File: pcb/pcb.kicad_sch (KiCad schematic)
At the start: 7 parts

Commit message: Start schematic
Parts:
- removed C? (x2): 100n, Capacitor_SMD:C_0603_1608Metric, symbol Device:C
- removed C? (x2): 22u, Capacitor_SMD:CP_Elec_4x3.9, symbol Device:C_Polarized_Small
- removed J?: EURO_PWR_2x5, Connector_IDC:IDC-Header_2x05_P2.54mm_Vertical, symbol eurocad:EURO_PWR_2x5
- removed R? (x2): 22R, Resistor_SMD:R_0603_1608Metric, symbol Device:R
- added C10, C12, C4, C5, C9: 100n, Capacitor_SMD:C_0603_1608Metric, symbol Device:C
- added C11, C13, C2, C3, C6: 10u, Capacitor_SMD:C_0805_2012Metric, symbol Device:C
- added C14, C16: 1n, Capacitor_SMD:C_0603_1608Metric, symbol Device:C
- added C15, C17: 100p, Capacitor_SMD:C_0603_1608Metric, symbol Device:C
- added C7, C8: 2.2u, Capacitor_SMD:C_0805_2012Metric, symbol Device:C
- added D1, D2: 1N5819, Diode_SMD:D_SOD-123, symbol Diode:1N5819
- added D10, D11, D12, D13, D14, D15, D16, D17, D18, D3, D4, D5, D6, D7, D8, D9: BAT54J, Diode_SMD:D_SOD-323F, symbol Diode:BAT54J
- added FB1: BLM21PG600SN1D, Inductor_SMD:L_0805_2012Metric, symbol Device:FerriteBead
- added J1, J10, J11, J2, J3, J5, J6, J7, J8, J9: PJ301M-12, Eurocad:PJ301M-12, symbol eurocad:PJ301M-12
- added J4: EURO_PWR_2x5, Eurocad:Eurorack_Power_Header, symbol eurocad:EURO_PWR_2x5
- added R10, R12, R14, R16, R18, R20, R6, R8: 100K, Resistor_SMD:R_0603_1608Metric, symbol Device:R
- added R11, R13, R15, R17, R19, R21, R25, R29, R7, R9: 1K, Resistor_SMD:R_0603_1608Metric, symbol Device:R
- added R22, R26: 2K2, Resistor_SMD:R_0603_1608Metric, symbol Device:R
- added R23, R27: 10K, Resistor_SMD:R_0603_1608Metric, symbol Device:R
- added R24, R28: 33K, Resistor_SMD:R_0603_1608Metric, symbol Device:R
- added SW1: RotaryEncoder_Switch, Rotary_Encoder:RotaryEncoder_Bourns_Horizontal_PEC09-2xxxF-Nxxxx, symbol Device:RotaryEncoder_Switch
- added U1: PCM5102, Package_SO:TSSOP-20_4.4x6.5mm_P0.65mm, symbol Audio:PCM5102
- added U2: TL072, Package_SO:SOIC-8_3.9x4.9mm_P1.27mm, symbol Amplifier_Operational:TL072
- added U6: Pico, MCU_RaspberryPi_and_Boards:RPi_Pico_SMD_TH, symbol MCU_RaspberryPi_and_Boards:Pico
- added U7: AZ1117-5.0, Package_TO_SOT_SMD:SOT-223-3_TabPin2, symbol Regulator_Linear:AZ1117-5.0
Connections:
- net +12V: now also C2.1, C4.1, D1.1 (K), U2.8 (V+), U7.3 (VI)
- net -12V: now also C3.2, C5.2, D2.2 (A), U2.4 (V-)
- net GND: now also C10.2, C11.2, C12.2, C13.2, C14.2, C16.2, C2.2, C3.1, C4.2, C5.1, C6.2, C8.2, C9.2, D10.2 (A), D12.2 (A), D14.2 (A), D16.2 (A), D18.2 (A), D3.2 (A), D6.2 (A), D8.2 (A), J1.1, J10.1, J11.1, J2.1, J3.1, J4.3 (GND), J4.4 (GND), J4.5 (GND), J4.6 (GND), J4.7 (GND), J4.8 (GND), J5.1, J6.1, J7.1, J8.1, J9.1, R10.1, R12.1, R14.1, R16.1, R18.1, R20.1, R6.1, R8.1, U1.10 (DEMP), U1.11 (FLT), U1.12 (SCK), U1.16 (FMT), U1.19 (DGND), U1.3 (CPGND), U1.9 (AGND), U2.3 (+), U2.5 (+), U6.13 (GND), U6.18 (GND), U6.23 (GND), U6.28 (GND), U6.3 (GND), U6.33 (AGND), U6.38 (GND), U6.42 (GND), U6.8 (GND), U7.1 (GND)
- new net: J2.3, R8.2, R9.2
- new net: C7.1, U1.2 (CAPP)
- new net: C7.2, U1.4 (CAPM)
- new net: C10.1, C11.1, FB1.2, U1.1 (CPVDD), U1.8 (AVDD)
- new net: J8.3, R18.2, R19.2
- new net: J7.3, R16.2, R17.2
- new net: C17.1, R27.1, R28.2, U2.6 (-)
- new net: C17.2, R28.1, R29.2, U2.7
- new net: C9.1, U1.18 (LDOO)
- new net: C8.1, U1.5 (VNEG)
- new net: J6.3, R14.2, R15.2
- new net: J3.3, R10.2, R11.2
- new net: J9.3, R20.2, R21.2
- new net: D1.2 (A), J4.1 (+12V), J4.2 (+12V)
- new net: D2.1 (K), J4.10 (-12V), J4.9 (-12V)
- new net: J5.3, R12.2, R13.2
- new net: C15.2, R24.1, R25.2, U2.1
- new net: C15.1, R23.1, R24.2, U2.2 (-)
- new net: C14.1, R22.1, R23.2
- new net: J11.3, R29.1
- new net: J10.3, R25.1
- new net: C16.1, R26.1, R27.2
- new net: J1.3, R6.2, R7.2
- new net +3V3: C12.1, C13.1, D11.1 (K), D13.1 (K), D15.1 (K), D17.1 (K), D4.1 (K), D5.1 (K), D7.1 (K), D9.1 (K), FB1.1, U1.20 (DVDD), U6.36 (3V3)
- new net +5V: C6.1, U6.39 (VSYS), U7.2 (VO)
- new net GPIO26: U1.14 (DIN), U6.31 (GPIO26_ADC0)
- new net GPIO27: U1.13 (BCK), U6.32 (GPIO27_ADC1)
- new net GPIO28: U1.15 (LRCK), U6.34 (GPIO28_ADC2)
- new net L: R22.2, U1.6 (OUTL)
- new net R: R26.2, U1.7 (OUTR)
- new net TRIGGER 1: D3.1 (K), D4.2 (A), R7.1
- new net TRIGGER 2: D5.2 (A), D6.1 (K), R9.1
- new net TRIGGER 3: D7.2 (A), D8.1 (K), R11.1
- new net TRIGGER 4: D10.1 (K), D9.2 (A), R13.1
- new net TRIGGER 5: D11.2 (A), D12.1 (K), R15.1
- new net TRIGGER 6: D13.2 (A), D14.1 (K), R17.1
- new net TRIGGER 7: D15.2 (A), D16.1 (K), R19.1
- new net TRIGGER 8: D17.2 (A), D18.1 (K), R21.1
- no-connect marks 0 -> 10

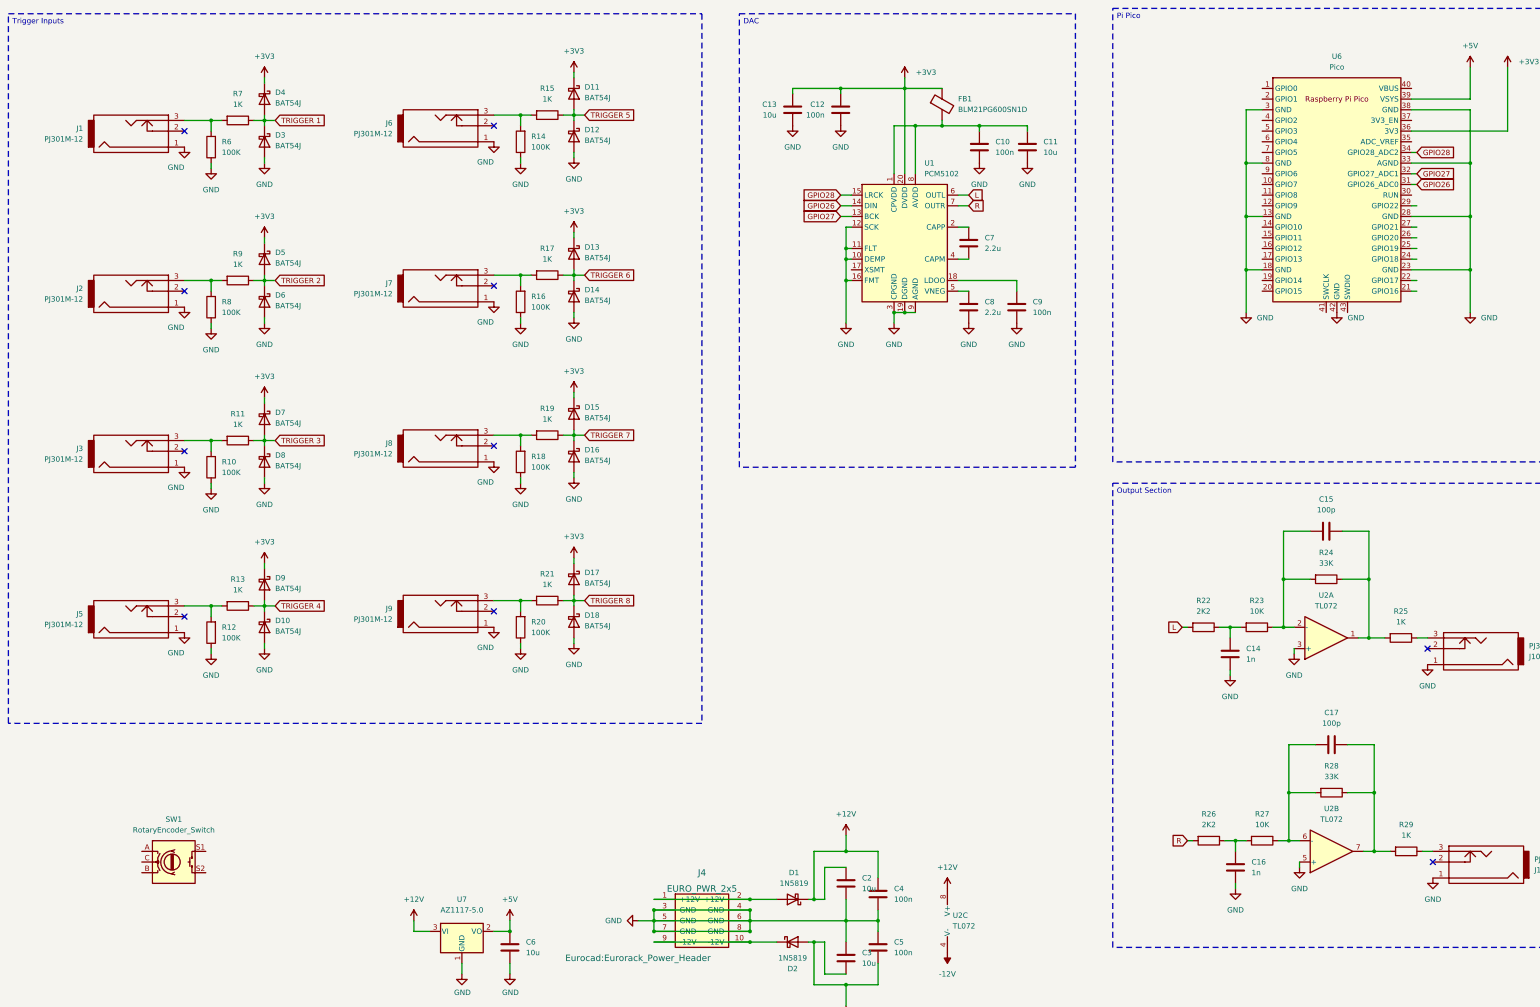
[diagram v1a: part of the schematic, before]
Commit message: Continue schematic
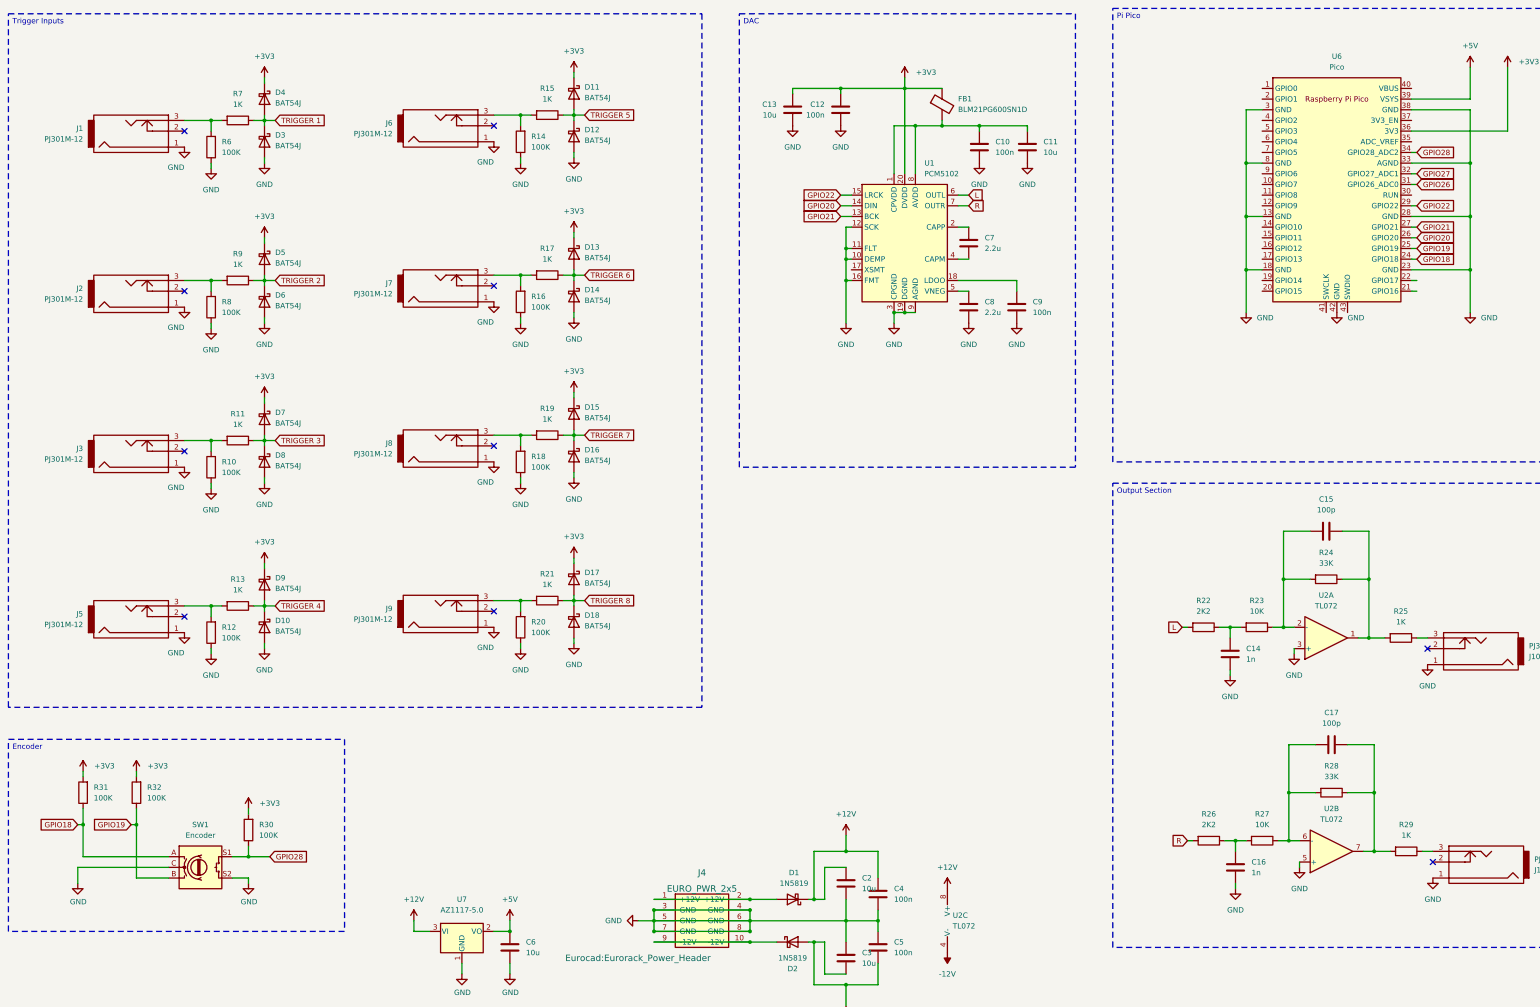
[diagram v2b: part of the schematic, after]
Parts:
- added R30, R31, R32: 100K, Resistor_SMD:R_0603_1608Metric, symbol Device:R
- SW1: value RotaryEncoder_Switch -> Encoder
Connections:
- net +3V3: now also R30.2, R31.2, R32.2
- net GND: now also SW1.C, SW1.S2
- net GPIO26: no longer U1.14 (DIN)
- net GPIO27: no longer U1.13 (BCK)
- net GPIO28: now also SW1.S1, R30.1; no longer U1.15 (LRCK)
- net GPIO18: now reaches U6.24 (GPIO18)
- net GPIO18: now also SW1.A, R31.1
- net GPIO19: now reaches U6.25 (GPIO19)
- net GPIO19: now also SW1.B, R32.1
- net GPIO20: now reaches U6.26 (GPIO20)
- net GPIO20: now also U1.14 (DIN)
- net GPIO21: now reaches U6.27 (GPIO21)
- net GPIO21: now also U1.13 (BCK)
- net GPIO22: now reaches U6.29 (GPIO22)
- net GPIO22: now also U1.15 (LRCK)
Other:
- moved on the sheet: SW1
